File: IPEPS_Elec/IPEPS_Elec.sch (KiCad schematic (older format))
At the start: 35 parts

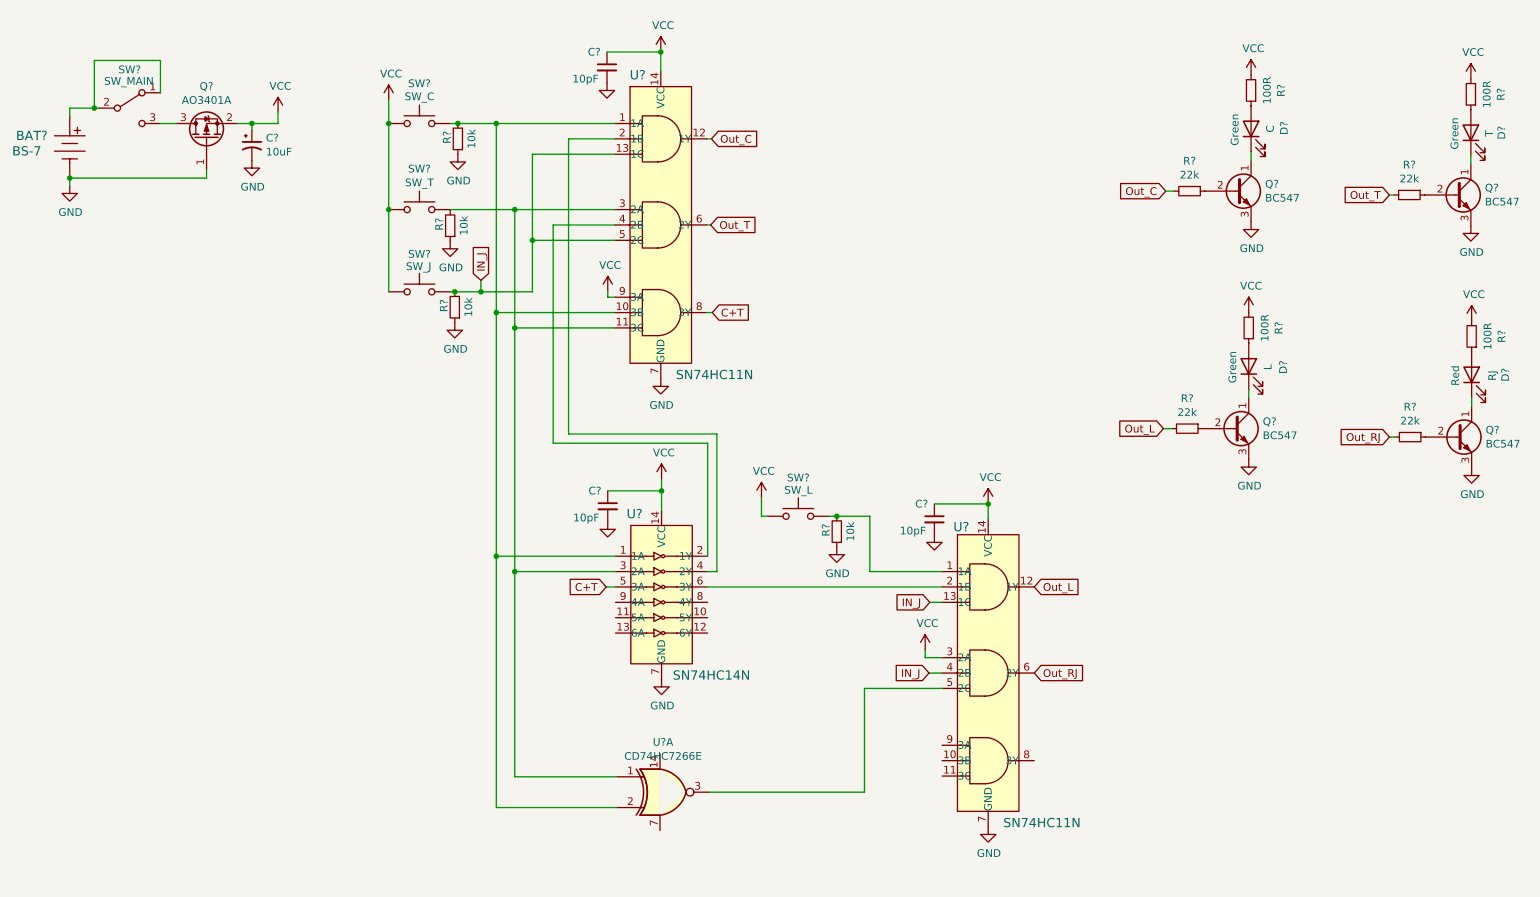
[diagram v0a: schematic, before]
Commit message: reorganise components
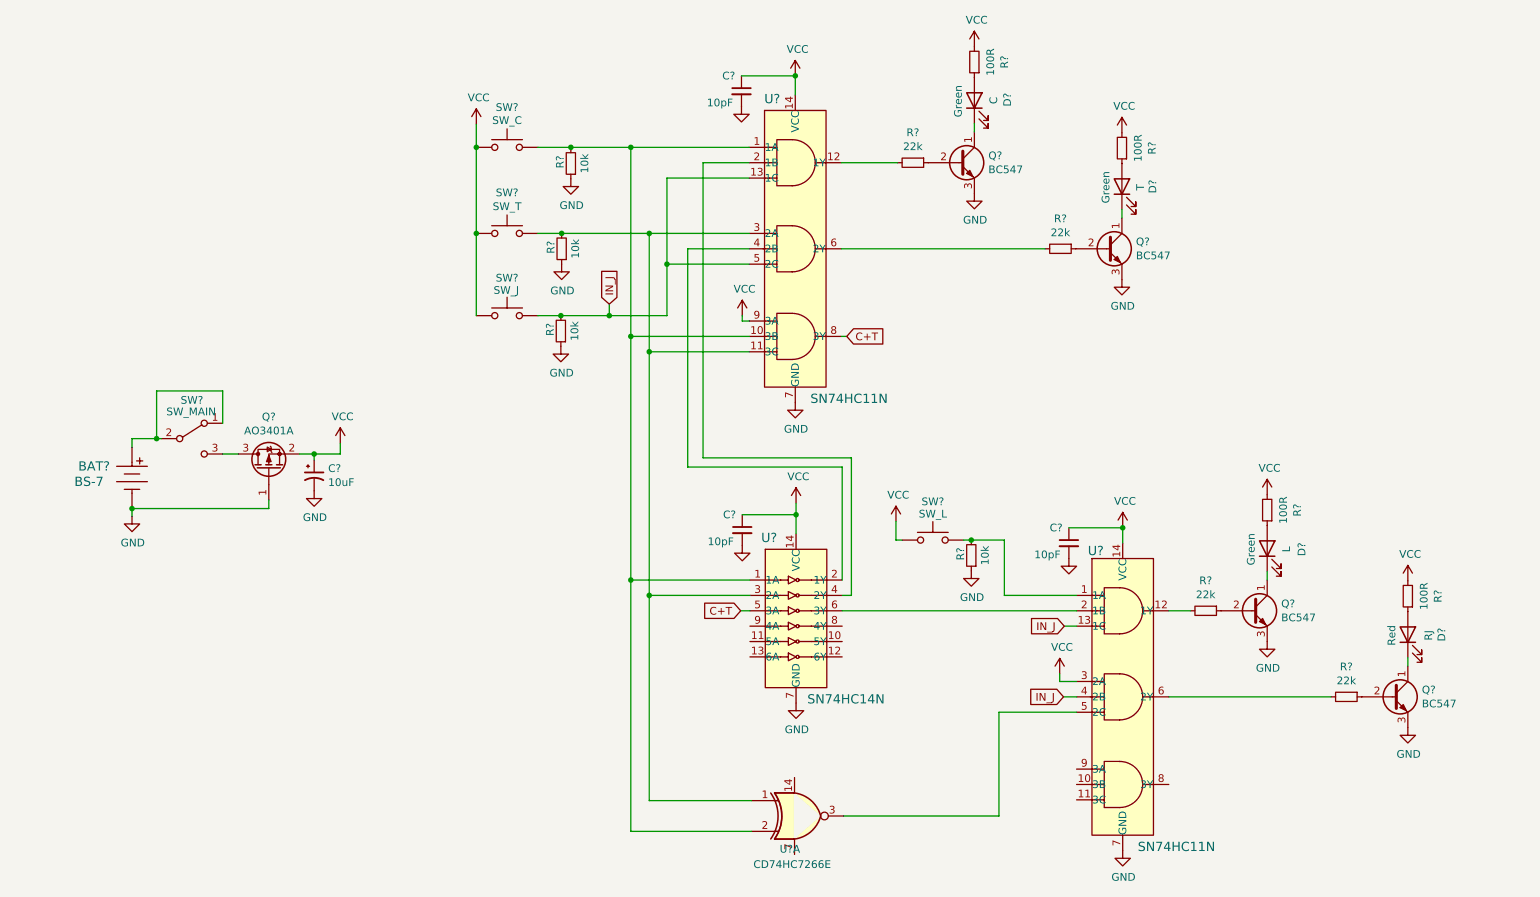
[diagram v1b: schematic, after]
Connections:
- net at SW?.2, U?.1, U?.11 (3C)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: now also R?.2
- net Out_C: no longer names the net of R?.2, U?.12 (1Y)
- net Out_L: no longer names the net of R?.2, U?.12 (1Y)
- net Out_RJ: no longer names the net of R?.2, U?.6 (2Y)
- net Out_T: no longer names the net of R?.2, U?.6 (2Y)
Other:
- moved on the sheet: BAT?, C?, D?, Q?, R?, SW?, U?, U?A
